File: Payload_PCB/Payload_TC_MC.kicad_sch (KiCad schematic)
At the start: 9 parts, among them U3 MCP9601-E/MX

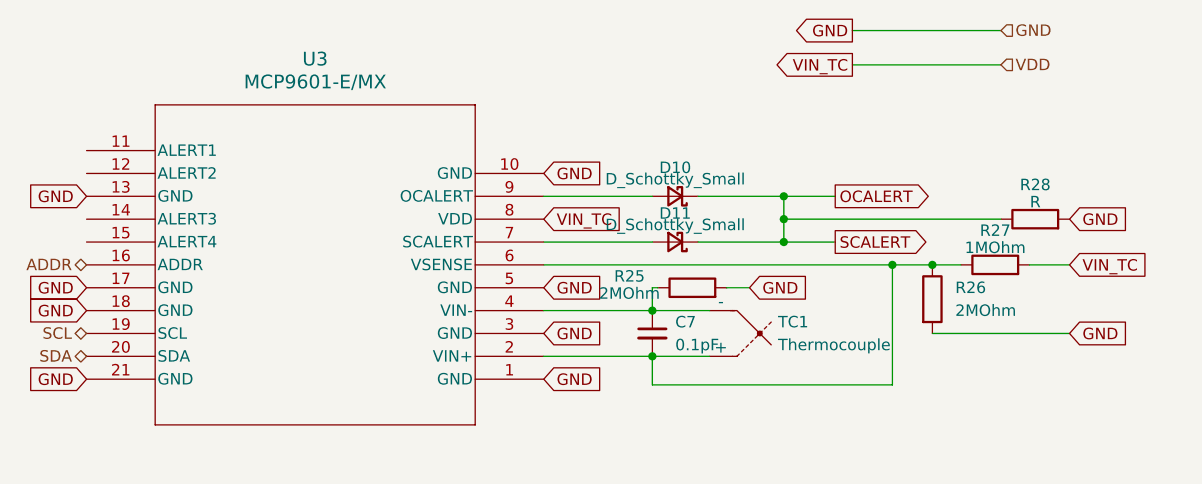
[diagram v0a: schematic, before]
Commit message: Added some actual parts
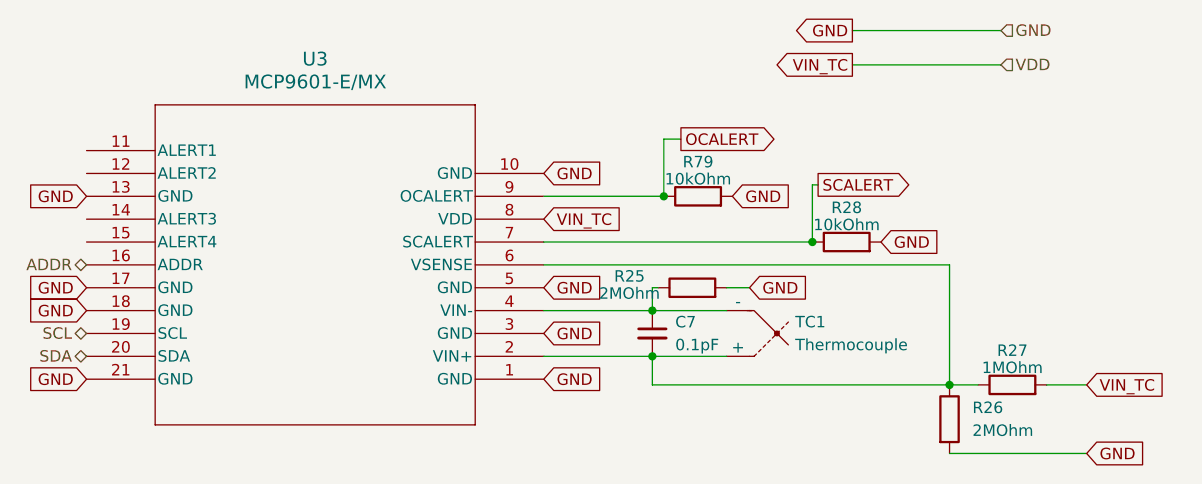
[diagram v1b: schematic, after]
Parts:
- removed D10, D11: D_Schottky_Small, symbol Device:D_Schottky_Small
- added R79: 10kOhm, symbol Device:R
- R28: value R -> 10kOhm
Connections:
- net GND: now also R79.2
- net OCALERT: now also U3.9 (OCALERT), R79.1; no longer R28.1
- net SCALERT: now reaches U3.7 (SCALERT)
- net SCALERT: now also R28.1
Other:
- company: (none) -> SpaceTeam Aachen
- title: (none) -> Thermocouple Microchip
- moved on the sheet: R26, R27, R28, TC1
